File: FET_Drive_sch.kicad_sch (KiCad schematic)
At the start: 15 parts, among them Q15 S8550, Q16 S8050_SMD, Q17 S8050_SMD, Q18 S8050_SMD

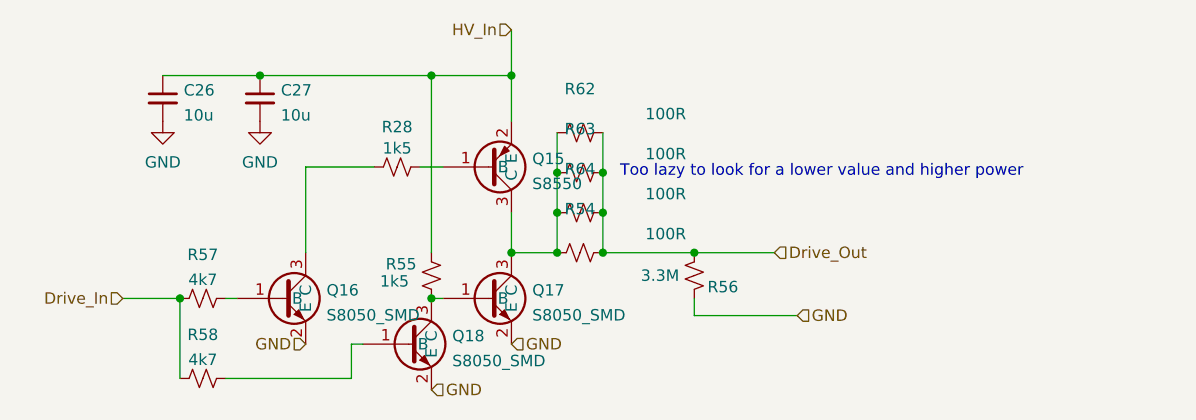
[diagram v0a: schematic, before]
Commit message: potential new version. Still to do Silkscreen and resistor value confirmations
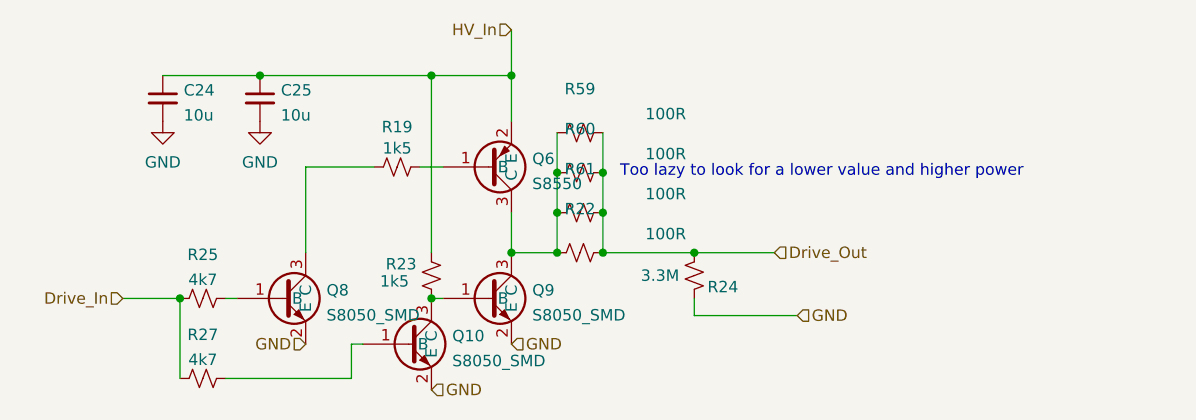
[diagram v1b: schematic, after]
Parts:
- renumbered C26 to C24, C27 to C25, Q18 to Q10, Q15 to Q6, Q16 to Q8, Q17 to Q9, R28 to R19, R54 to R22, R55 to R23, R56 to R24, R57 to R25, R58 to R27, R62 to R59, R63 to R60, R64 to R61
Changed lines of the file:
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@@
   (symbol (lib_id "Device:R_Small_US") (at 168.275 84.455 0) (mirror y)
     (in_bom yes) (on_board yes)
-    (property "Reference" "R56" (id 0) (at 171.45 85.725 0))
+    (property "Reference" "R24" (id 0) (at 171.45 85.725 0))
     (property "Value" "3.3M" (id 1) (at 164.465 84.455 0))
     (property "Footprint" "Resistor_SMD:R_0402_1005Metric" (id 2) (at 168.275 84.455 0)
@@
   (symbol (lib_id "Device:R_Small_US") (at 113.665 86.995 90)
     (in_bom yes) (on_board yes)
-    (property "Reference" "R57" (id 0) (at 113.665 82.1395 90))
+    (property "Reference" "R25" (id 0) (at 113.665 82.1395 90))
     (property "Value" "4k7" (id 1) (at 113.665 84.9146 90))
     (property "Footprint" "Resistor_SMD:R_0402_1005Metric" (id 2) (at 113.665 86.995 0)
@@
   (symbol (lib_id "Device:C_Small") (at 120.015 64.77 0)
     (in_bom yes) (on_board yes) (fields_autoplaced)
-    (property "Reference" "C27" (id 0) (at 122.3391 63.8678 0)
+    (property "Reference" "C25" (id 0) (at 122.3391 63.8678 0)
       (effects (font (size 1.27 1.27)) (justify left))
     )
@@
   (symbol (lib_id "MyDevices:S8050_SMD") (at 137.795 92.075 0)
     (in_bom yes) (on_board yes) (fields_autoplaced)
-    (property "Reference" "Q18" (id 0) (at 141.3764 91.1665 0)
+    (property "Reference" "Q10" (id 0) (at 141.3764 91.1665 0)
       (effects (font (size 1.27 1.27)) (justify left))
     )
@@
   (symbol (lib_id "Device:R_Small_US") (at 155.575 68.58 90)
     (in_bom yes) (on_board yes)
-    (property "Reference" "R62" (id 0) (at 155.575 63.7245 90))
+    (property "Reference" "R59" (id 0) (at 155.575 63.7245 90))
     (property "Value" "100R" (id 1) (at 165.1 66.4996 90))
     (property "Footprint" "Resistor_SMD:R_0402_1005Metric" (id 2) (at 155.575 68.58 0)
@@
   (symbol (lib_id "MyDevices:S8050_SMD") (at 146.685 86.995 0)
     (in_bom yes) (on_board yes) (fields_autoplaced)
-    (property "Reference" "Q17" (id 0) (at 150.2664 86.0865 0)
+    (property "Reference" "Q9" (id 0) (at 150.2664 86.0865 0)
       (effects (font (size 1.27 1.27)) (justify left))
     )
@@
   (symbol (lib_id "Device:R_Small_US") (at 155.575 81.915 90)
     (in_bom yes) (on_board yes)
-    (property "Reference" "R54" (id 0) (at 155.575 77.0595 90))
+    (property "Reference" "R22" (id 0) (at 155.575 77.0595 90))
     (property "Value" "100R" (id 1) (at 165.1 79.8346 90))
     (property "Footprint" "Resistor_SMD:R_0402_1005Metric" (id 2) (at 155.575 81.915 0)
@@
   (symbol (lib_id "Device:R_Small_US") (at 135.255 72.39 90)
     (in_bom yes) (on_board yes)
-    (property "Reference" "R28" (id 0) (at 135.255 67.945 90))
+    (property "Reference" "R19" (id 0) (at 135.255 67.945 90))
     (property "Value" "1k5" (id 1) (at 135.255 70.3096 90))
     (property "Footprint" "Resistor_SMD:R_0402_1005Metric" (id 2) (at 135.255 72.39 0)
@@
   (symbol (lib_id "Device:R_Small_US") (at 139.065 84.455 180)
     (in_bom yes) (on_board yes)
-    (property "Reference" "R55" (id 0) (at 133.985 83.185 0)
+    (property "Reference" "R23" (id 0) (at 133.985 83.185 0)
       (effects (font (size 1.27 1.27)) (justify right))
     )
@@
   (symbol (lib_id "MyDevices:S8550") (at 146.685 72.39 0)
     (in_bom yes) (on_board yes) (fields_autoplaced)
-    (property "Reference" "Q15" (id 0) (at 150.2664 71.4815 0)
+    (property "Reference" "Q6" (id 0) (at 150.2664 71.4815 0)
       (effects (font (size 1.27 1.27)) (justify left))
     )
@@
   (symbol (lib_id "Device:C_Small") (at 109.22 64.77 0)
     (in_bom yes) (on_board yes) (fields_autoplaced)
-    (property "Reference" "C26" (id 0) (at 111.5441 63.8678 0)
+    (property "Reference" "C24" (id 0) (at 111.5441 63.8678 0)
       (effects (font (size 1.27 1.27)) (justify left))
     )
@@
   (symbol (lib_id "power:GND") (at 109.22 67.31 0)
     (in_bom yes) (on_board yes) (fields_autoplaced)
-    (property "Reference" "#PWR0117" (id 0) (at 109.22 73.66 0)
+    (property "Reference" "#PWR0113" (id 0) (at 109.22 73.66 0)
       (effects (font (size 1.27 1.27)) hide)
     )
@@
   (symbol (lib_id "MyDevices:S8050_SMD") (at 123.825 86.995 0)
     (in_bom yes) (on_board yes) (fields_autoplaced)
-    (property "Reference" "Q16" (id 0) (at 127.4064 86.0865 0)
+    (property "Reference" "Q8" (id 0) (at 127.4064 86.0865 0)
       (effects (font (size 1.27 1.27)) (justify left))
     )
@@
   (symbol (lib_id "power:GND") (at 120.015 67.31 0)
     (in_bom yes) (on_board yes) (fields_autoplaced)
-    (property "Reference" "#PWR0115" (id 0) (at 120.015 73.66 0)
+    (property "Reference" "#PWR0111" (id 0) (at 120.015 73.66 0)
       (effects (font (size 1.27 1.27)) hide)
     )
@@
   (symbol (lib_id "Device:R_Small_US") (at 155.575 77.47 90)
     (in_bom yes) (on_board yes)
-    (property "Reference" "R64" (id 0) (at 155.575 72.6145 90))
+    (property "Reference" "R61" (id 0) (at 155.575 72.6145 90))
     (property "Value" "100R" (id 1) (at 165.1 75.3896 90))
     (property "Footprint" "Resistor_SMD:R_0402_1005Metric" (id 2) (at 155.575 77.47 0)
@@
   (symbol (lib_id "Device:R_Small_US") (at 113.665 95.885 90)
     (in_bom yes) (on_board yes)
-    (property "Reference" "R58" (id 0) (at 113.665 91.0295 90))
+    (property "Reference" "R27" (id 0) (at 113.665 91.0295 90))
     (property "Value" "4k7" (id 1) (at 113.665 93.8046 90))
     (property "Footprint" "Resistor_SMD:R_0402_1005Metric" (id 2) (at 113.665 95.885 0)
@@
   (symbol (lib_id "Device:R_Small_US") (at 155.575 73.025 90)
     (in_bom yes) (on_board yes)
-    (property "Reference" "R63" (id 0) (at 155.575 68.1695 90))
+    (property "Reference" "R60" (id 0) (at 155.575 68.1695 90))
     (property "Value" "100R" (id 1) (at 165.1 70.9446 90))
     (property "Footprint" "Resistor_SMD:R_0402_1005Metric" (id 2) (at 155.575 73.025 0)

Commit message: hadnt saved... this is the last commit message
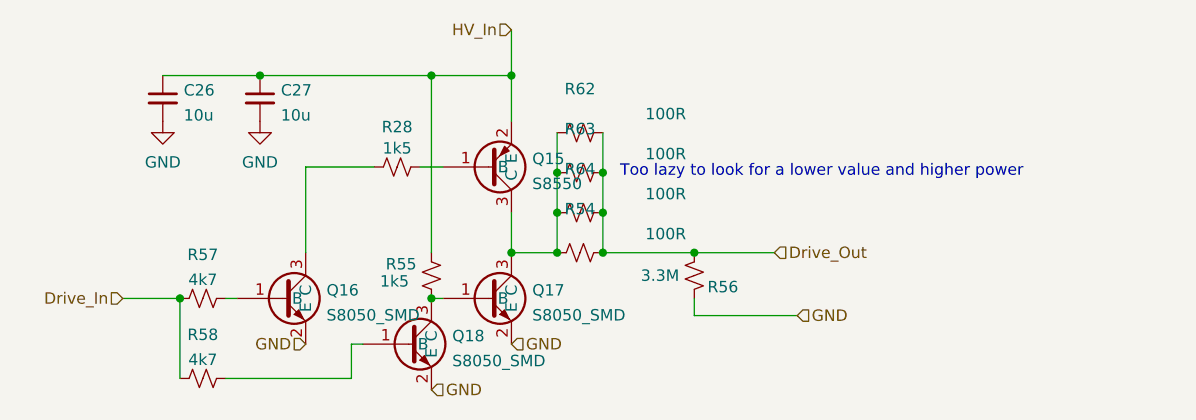
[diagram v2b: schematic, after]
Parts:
- renumbered C24 to C26, C25 to C27, Q6 to Q15, Q8 to Q16, Q9 to Q17, Q10 to Q18, R19 to R28, R22 to R54, R23 to R55, R24 to R56, R25 to R57, R27 to R58, R59 to R62, R60 to R63, R61 to R64
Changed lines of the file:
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@@
   (symbol (lib_id "Device:R_Small_US") (at 168.275 84.455 0) (mirror y)
     (in_bom yes) (on_board yes)
-    (property "Reference" "R24" (id 0) (at 171.45 85.725 0))
+    (property "Reference" "R56" (id 0) (at 171.45 85.725 0))
     (property "Value" "3.3M" (id 1) (at 164.465 84.455 0))
     (property "Footprint" "Resistor_SMD:R_0402_1005Metric" (id 2) (at 168.275 84.455 0)
@@
   (symbol (lib_id "Device:R_Small_US") (at 113.665 86.995 90)
     (in_bom yes) (on_board yes)
-    (property "Reference" "R25" (id 0) (at 113.665 82.1395 90))
+    (property "Reference" "R57" (id 0) (at 113.665 82.1395 90))
     (property "Value" "4k7" (id 1) (at 113.665 84.9146 90))
     (property "Footprint" "Resistor_SMD:R_0402_1005Metric" (id 2) (at 113.665 86.995 0)
@@
   (symbol (lib_id "Device:C_Small") (at 120.015 64.77 0)
     (in_bom yes) (on_board yes) (fields_autoplaced)
-    (property "Reference" "C25" (id 0) (at 122.3391 63.8678 0)
+    (property "Reference" "C27" (id 0) (at 122.3391 63.8678 0)
       (effects (font (size 1.27 1.27)) (justify left))
     )
@@
   (symbol (lib_id "MyDevices:S8050_SMD") (at 137.795 92.075 0)
     (in_bom yes) (on_board yes) (fields_autoplaced)
-    (property "Reference" "Q10" (id 0) (at 141.3764 91.1665 0)
+    (property "Reference" "Q18" (id 0) (at 141.3764 91.1665 0)
       (effects (font (size 1.27 1.27)) (justify left))
     )
@@
   (symbol (lib_id "Device:R_Small_US") (at 155.575 68.58 90)
     (in_bom yes) (on_board yes)
-    (property "Reference" "R59" (id 0) (at 155.575 63.7245 90))
+    (property "Reference" "R62" (id 0) (at 155.575 63.7245 90))
     (property "Value" "100R" (id 1) (at 165.1 66.4996 90))
     (property "Footprint" "Resistor_SMD:R_0402_1005Metric" (id 2) (at 155.575 68.58 0)
@@
   (symbol (lib_id "MyDevices:S8050_SMD") (at 146.685 86.995 0)
     (in_bom yes) (on_board yes) (fields_autoplaced)
-    (property "Reference" "Q9" (id 0) (at 150.2664 86.0865 0)
+    (property "Reference" "Q17" (id 0) (at 150.2664 86.0865 0)
       (effects (font (size 1.27 1.27)) (justify left))
     )
@@
   (symbol (lib_id "Device:R_Small_US") (at 155.575 81.915 90)
     (in_bom yes) (on_board yes)
-    (property "Reference" "R22" (id 0) (at 155.575 77.0595 90))
+    (property "Reference" "R54" (id 0) (at 155.575 77.0595 90))
     (property "Value" "100R" (id 1) (at 165.1 79.8346 90))
     (property "Footprint" "Resistor_SMD:R_0402_1005Metric" (id 2) (at 155.575 81.915 0)
@@
   (symbol (lib_id "Device:R_Small_US") (at 135.255 72.39 90)
     (in_bom yes) (on_board yes)
-    (property "Reference" "R19" (id 0) (at 135.255 67.945 90))
+    (property "Reference" "R28" (id 0) (at 135.255 67.945 90))
     (property "Value" "1k5" (id 1) (at 135.255 70.3096 90))
     (property "Footprint" "Resistor_SMD:R_0402_1005Metric" (id 2) (at 135.255 72.39 0)
@@
   (symbol (lib_id "Device:R_Small_US") (at 139.065 84.455 180)
     (in_bom yes) (on_board yes)
-    (property "Reference" "R23" (id 0) (at 133.985 83.185 0)
+    (property "Reference" "R55" (id 0) (at 133.985 83.185 0)
       (effects (font (size 1.27 1.27)) (justify right))
     )
@@
   (symbol (lib_id "MyDevices:S8550") (at 146.685 72.39 0)
     (in_bom yes) (on_board yes) (fields_autoplaced)
-    (property "Reference" "Q6" (id 0) (at 150.2664 71.4815 0)
+    (property "Reference" "Q15" (id 0) (at 150.2664 71.4815 0)
       (effects (font (size 1.27 1.27)) (justify left))
     )
@@
   (symbol (lib_id "Device:C_Small") (at 109.22 64.77 0)
     (in_bom yes) (on_board yes) (fields_autoplaced)
-    (property "Reference" "C24" (id 0) (at 111.5441 63.8678 0)
+    (property "Reference" "C26" (id 0) (at 111.5441 63.8678 0)
       (effects (font (size 1.27 1.27)) (justify left))
     )
@@
   (symbol (lib_id "power:GND") (at 109.22 67.31 0)
     (in_bom yes) (on_board yes) (fields_autoplaced)
-    (property "Reference" "#PWR0113" (id 0) (at 109.22 73.66 0)
+    (property "Reference" "#PWR0117" (id 0) (at 109.22 73.66 0)
       (effects (font (size 1.27 1.27)) hide)
     )
@@
   (symbol (lib_id "MyDevices:S8050_SMD") (at 123.825 86.995 0)
     (in_bom yes) (on_board yes) (fields_autoplaced)
-    (property "Reference" "Q8" (id 0) (at 127.4064 86.0865 0)
+    (property "Reference" "Q16" (id 0) (at 127.4064 86.0865 0)
       (effects (font (size 1.27 1.27)) (justify left))
     )
@@
   (symbol (lib_id "power:GND") (at 120.015 67.31 0)
     (in_bom yes) (on_board yes) (fields_autoplaced)
-    (property "Reference" "#PWR0111" (id 0) (at 120.015 73.66 0)
+    (property "Reference" "#PWR0115" (id 0) (at 120.015 73.66 0)
       (effects (font (size 1.27 1.27)) hide)
     )
@@
   (symbol (lib_id "Device:R_Small_US") (at 155.575 77.47 90)
     (in_bom yes) (on_board yes)
-    (property "Reference" "R61" (id 0) (at 155.575 72.6145 90))
+    (property "Reference" "R64" (id 0) (at 155.575 72.6145 90))
     (property "Value" "100R" (id 1) (at 165.1 75.3896 90))
     (property "Footprint" "Resistor_SMD:R_0402_1005Metric" (id 2) (at 155.575 77.47 0)
@@
   (symbol (lib_id "Device:R_Small_US") (at 113.665 95.885 90)
     (in_bom yes) (on_board yes)
-    (property "Reference" "R27" (id 0) (at 113.665 91.0295 90))
+    (property "Reference" "R58" (id 0) (at 113.665 91.0295 90))
     (property "Value" "4k7" (id 1) (at 113.665 93.8046 90))
     (property "Footprint" "Resistor_SMD:R_0402_1005Metric" (id 2) (at 113.665 95.885 0)
@@
   (symbol (lib_id "Device:R_Small_US") (at 155.575 73.025 90)
     (in_bom yes) (on_board yes)
-    (property "Reference" "R60" (id 0) (at 155.575 68.1695 90))
+    (property "Reference" "R63" (id 0) (at 155.575 68.1695 90))
     (property "Value" "100R" (id 1) (at 165.1 70.9446 90))
     (property "Footprint" "Resistor_SMD:R_0402_1005Metric" (id 2) (at 155.575 73.025 0)
